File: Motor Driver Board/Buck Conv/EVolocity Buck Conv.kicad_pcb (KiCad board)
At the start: 4 copper layers, 120 x 90 mm, 53 parts, among them J1 Screw_Terminal_01x02, J2 XT30, J3 Screw_Terminal_01x02, J4 Conn_01x04, U1 NRF24L01_Breakout, U2 LM2576HVT-5, U4 L298N

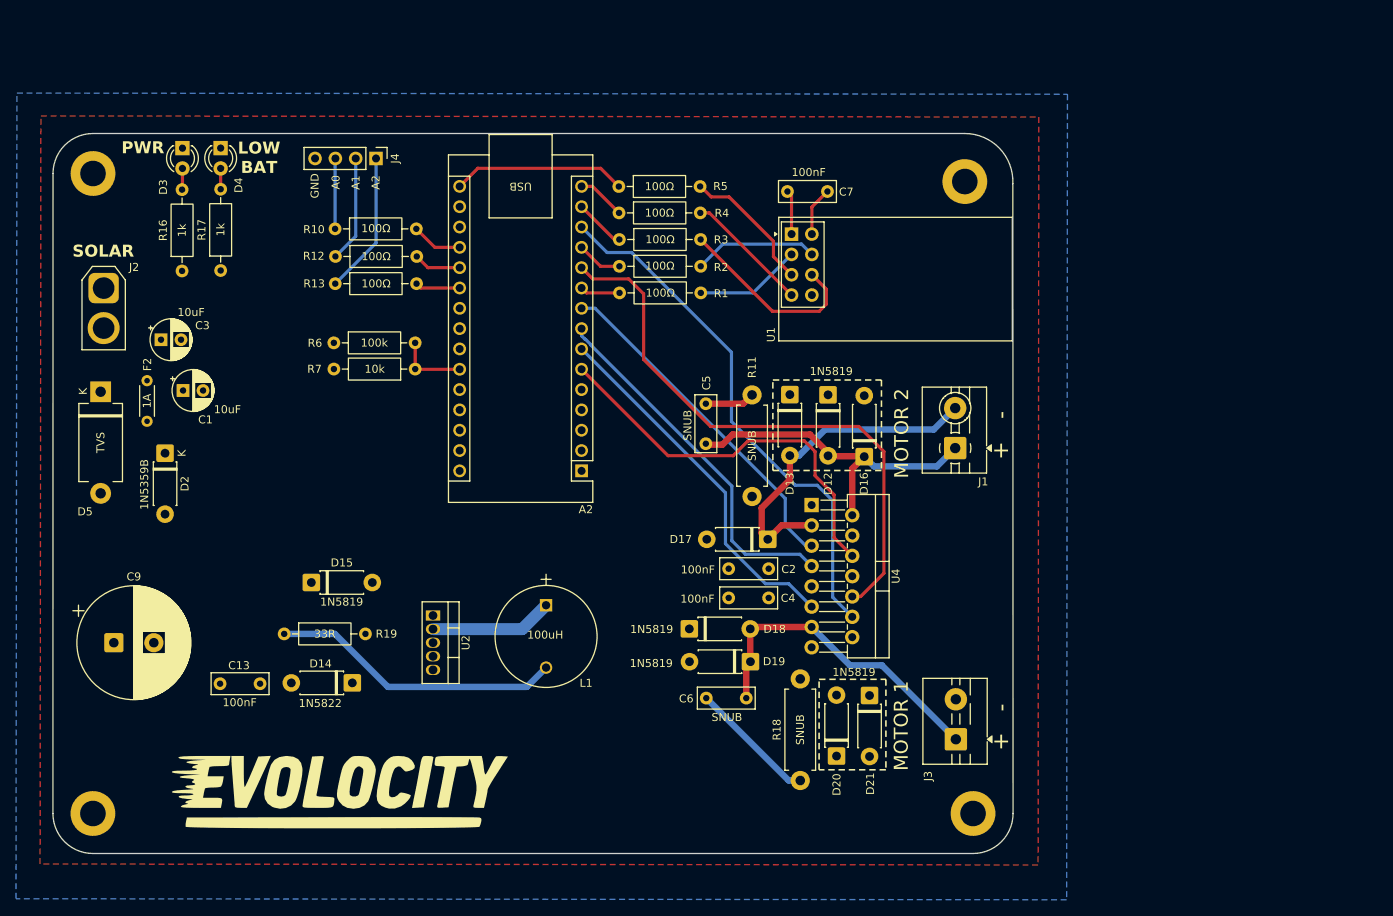
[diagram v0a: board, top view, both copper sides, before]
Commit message: updates after catchup
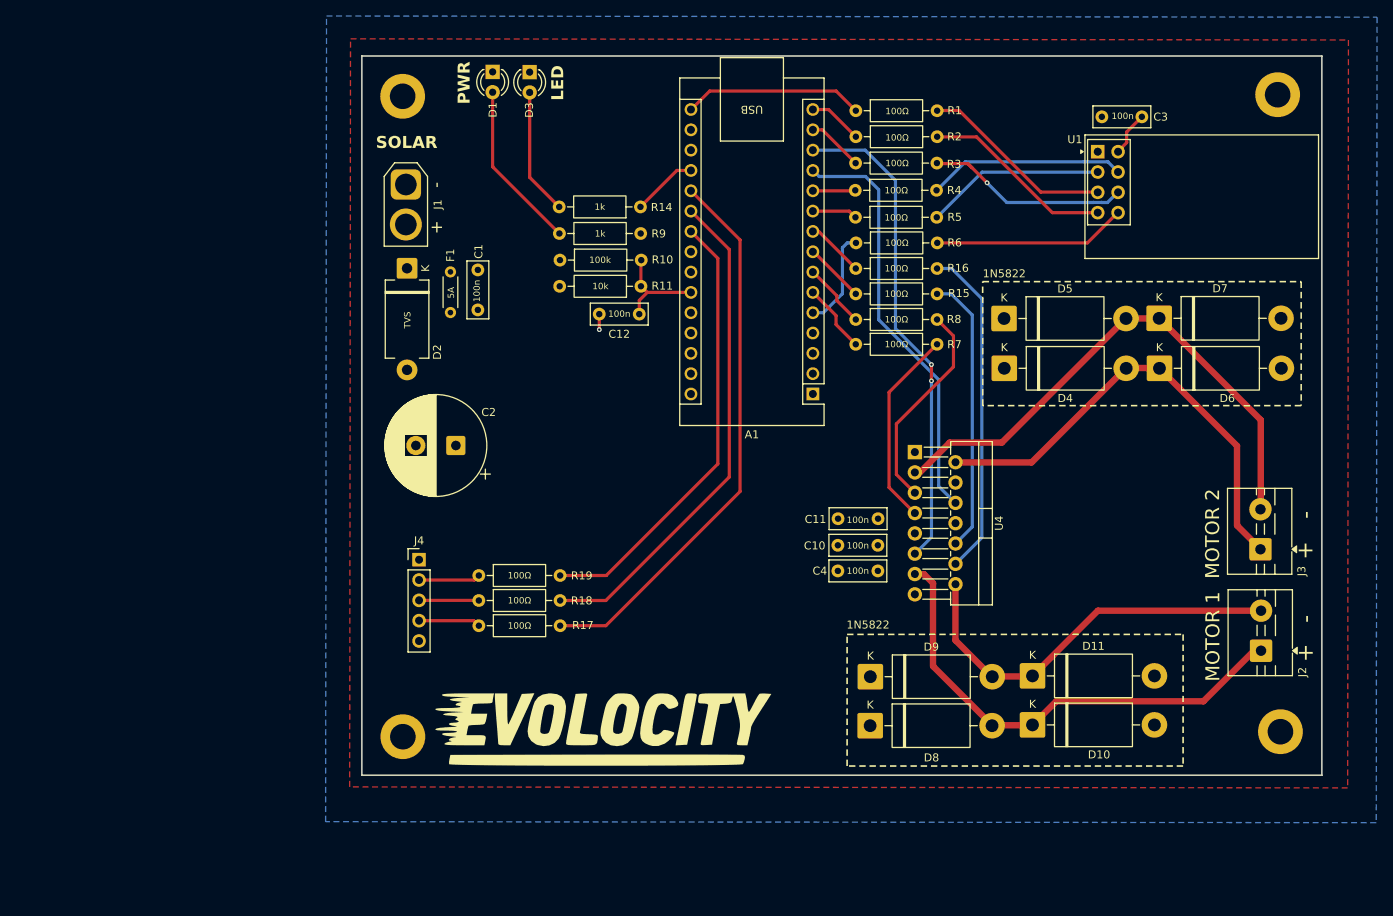
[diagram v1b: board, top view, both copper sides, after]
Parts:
- removed A2: Arduino_Nano_v3.x, Module:Arduino_Nano
- removed C13, C7: 100nF, Capacitor_THT:C_Rect_L7.0mm_W2.5mm_P5.00mm
- removed C5, C6: C_Snub, Capacitor_THT:C_Rect_L7.0mm_W2.5mm_P5.00mm
- removed C9: 100m, Capacitor_THT:CP_Radial_D14.0mm_P5.00mm
- removed D12, D13, D15, D16, D17, D18, D19, D20, D21: 1N5819, Diode_THT:D_DO-41_SOD81_P7.62mm_Horizontal
- removed D14: 1N5822, Diode_THT:D_DO-41_SOD81_P7.62mm_Horizontal
- removed F2: 1A, Resistor_THT:R_Axial_DIN0204_L3.6mm_D1.6mm_P5.08mm_Horizontal
- removed L1: 100uH, Library1:IND_BOURNS_RLB1314
- removed R12, R13: 100, Resistor_THT:R_Axial_DIN0207_L6.3mm_D2.5mm_P10.16mm_Horizontal
- removed U2: LM2576HVT-5, Package_TO_SOT_THT:TO-220-5_Vertical
- added A1: Arduino Nano, Module:Arduino_Nano, F.Cu at (136.0, 98.3)
- added C10: 100nF, Capacitor_THT:C_Rect_L7.0mm_W2.5mm_P5.00mm, F.Cu at (144.1, 117.2)
- added C11: 100nF, Capacitor_THT:C_Rect_L7.0mm_W2.5mm_P5.00mm, F.Cu at (144.1, 113.9)
- added C12: 100nF, Capacitor_THT:C_Rect_L7.0mm_W2.5mm_P5.00mm, F.Cu at (114.3, 88.3)
- added D1: Green, LED_THT:LED_D3.0mm_FlatTop, F.Cu at (96.0, 58.0)
- added D10: 1N5822, Diode_THT:D_DO-201AD_P15.24mm_Horizontal, F.Cu at (163.4, 139.7)
- added D11: 1N5822, Diode_THT:D_DO-201AD_P15.24mm_Horizontal, F.Cu at (163.4, 133.6)
- added D6: 1N5822, Diode_THT:D_DO-201AD_P15.24mm_Horizontal, F.Cu at (179.3, 95.1)
- added D7: 1N5822, Diode_THT:D_DO-201AD_P15.24mm_Horizontal, F.Cu at (179.3, 88.8)
- added D8: 1N5822, Diode_THT:D_DO-201AD_P15.24mm_Horizontal, F.Cu at (143.1, 139.8)
- added D9: 1N5822, Diode_THT:D_DO-201AD_P15.24mm_Horizontal, F.Cu at (143.2, 133.7)
- added F1: 5A, Resistor_THT:R_Axial_DIN0204_L3.6mm_D1.6mm_P5.08mm_Horizontal, F.Cu at (90.7, 83.0)
- added R14: 1k, Resistor_THT:R_Axial_DIN0207_L6.3mm_D2.5mm_P10.16mm_Horizontal, F.Cu at (114.4, 74.9)
- added R15: 100R, Resistor_THT:R_Axial_DIN0207_L6.3mm_D2.5mm_P10.16mm_Horizontal, F.Cu at (141.3, 85.8)
- added R8: 100R, Resistor_THT:R_Axial_DIN0207_L6.3mm_D2.5mm_P10.16mm_Horizontal, F.Cu at (141.3, 89.0)
- added R9: 1k, Resistor_THT:R_Axial_DIN0207_L6.3mm_D2.5mm_P10.16mm_Horizontal, F.Cu at (114.5, 78.2)
- C1, C3: value 10uF -> 100nF; footprint Capacitor_THT:CP_Radial_D5.0mm_P2.50mm -> Capacitor_THT:C_Rect_L7.0mm_W2.5mm_P5.00mm
- C2: value 100nF -> 470uF; footprint Capacitor_THT:C_Rect_L7.0mm_W2.5mm_P5.00mm -> Capacitor_THT:CP_Radial_D12.5mm_P5.00mm
- D2: value 1N5359B -> 1.5KE39CA (TVS); footprint Diode_THT:D_DO-41_SOD81_P7.62mm_Horizontal -> Diode_THT:D_DO-201_P12.70mm_Horizontal
- D4: value Red -> 1N5822; footprint LED_THT:LED_D3.0mm_FlatTop -> Diode_THT:D_DO-201AD_P15.24mm_Horizontal
- D5: value 1.5KE39CA (TVS) -> 1N5822; footprint Diode_THT:D_DO-201_P12.70mm_Horizontal -> Diode_THT:D_DO-201AD_P15.24mm_Horizontal
- J1: value Screw_Terminal_01x02 -> XT30; footprint TerminalBlock:TerminalBlock_MaiXu_MX126-5.0-02P_1x02_P5.00mm -> Connector_AMASS:AMASS_XT30U-F_1x02_P5.0mm_Vertical
- J2: value XT30 -> Screw_Terminal_01x02; footprint Connector_AMASS:AMASS_XT30U-F_1x02_P5.0mm_Vertical -> TerminalBlock:TerminalBlock_MaiXu_MX126-5.0-02P_1x02_P5.00mm
- J4: value Conn_01x04 -> Conn_01x05; footprint Connector_PinHeader_2.54mm:PinHeader_1x04_P2.54mm_Vertical -> Connector_PinHeader_2.54mm:PinHeader_1x05_P2.54mm_Vertical
- R1, R2, R3, R4, R5: value 100 -> 100R
- R10: value 100 -> 100k
- R11: value R_snub -> 10k; footprint Resistor_THT:R_Axial_DIN0411_L9.9mm_D3.6mm_P12.70mm_Horizontal -> Resistor_THT:R_Axial_DIN0207_L6.3mm_D2.5mm_P10.16mm_Horizontal
- R16, R17: value 1k -> 100R
- R18: value R_snub -> 100R; footprint Resistor_THT:R_Axial_DIN0411_L9.9mm_D3.6mm_P12.70mm_Horizontal -> Resistor_THT:R_Axial_DIN0207_L6.3mm_D2.5mm_P10.16mm_Horizontal
- R19: value 33R -> 100R
- R6: value 100k -> 100R
- R7: value 10k -> 100R
- moved J2 151.6 mm to (192.0, 130.4), turned to 90 degrees
- moved C3 125.7 mm to (177.1, 63.7), turned to 180 degrees
- moved D5 113.3 mm to (159.9, 88.9), turned to 0 degrees
- moved D4 101.7 mm to (159.9, 95.1), turned to 0 degrees
- moved H3 97.6 mm to (194.1, 60.9)
- moved R16 84.2 mm to (141.3, 82.6), turned to 0 degrees
- moved H4 79.3 mm to (194.4, 140.5)
- moved J1 76.2 mm to (85.1, 72.1), turned to -90 degrees
- moved R6 66.5 mm to (141.4, 79.4)
- moved R7 55.2 mm to (141.3, 92.1), turned to 0 degrees
- moved R17 54.9 mm to (94.2, 127.3), turned to 0 degrees
- moved J4 50.4 mm to (86.8, 119.0), turned to 0 degrees
- moved R18 46.1 mm to (94.2, 124.1), turned to 0 degrees
- moved J3 44.9 mm to (191.9, 117.7)
- moved D3 44.4 mm to (100.6, 58.1)
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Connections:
- C1 pad 1: +5V -> PowerInput+
- C2 pad 1: +5V -> PowerInput+
- C4 pad 1: +5V -> PowerInput+
- D2 pad 1: +5V -> PowerInput+
- D4 pad 1: GND -> PowerInput+
- D5 pad 1: Net-(D5-A1) -> PowerInput+
- D5 pad 2: GND -> Net-(D5-A)
- J1 pad 1: Net-(D12-A) -> GND
- J1 pad 2: Net-(D13-A) -> Net-(J1-Pin_2)
- J2 pad 1: GND -> Net-(D10-K)
- J2 pad 2: Net-(D5-A1) -> Net-(D11-K)
- J3 pad 1: Net-(D18-A) -> Net-(D4-A)
- J3 pad 2: Net-(D20-A) -> Net-(D5-A)
- J4 pad 1: /A2 -> GND
- J4 pad 2: /A1 -> /A3
- J4 pad 3: /A0 -> /A2
- J4 pad 4: GND -> /A1
- R1 pad 2: /Radio_CE -> /Radio_SCK
- R10 pad 1: /A0 -> PowerInput+
- R10 pad 2: Net-(A2-A0) -> /V_Panel_Analog
- R11 pad 1: Net-(C5-Pad2) -> /V_Panel_Analog
- R11 pad 2: Net-(D13-A) -> GND
- R16 pad 1: +5V -> Net-(A1-D6)
- R16 pad 2: Net-(D3-A) -> /Motor_IN4
- R17 pad 1: /LowBattLED -> /A1
- R17 pad 2: Net-(D4-A) -> Net-(A1-A1)
- R18 pad 1: Net-(C6-Pad2) -> /A2
- R18 pad 2: Net-(D20-A) -> Net-(A1-A2)
- R19 pad 1: Net-(L1-Pad2) -> /A3
- R2 pad 2: /Radio_CS -> /Radio_MISO
- R4 pad 2: /Radio_MISO -> /Radio_CS
- R5 pad 2: /Radio_SCK -> /Radio_CE
- R6 pad 1: +5V -> Net-(A1-D2)
- R6 pad 2: /V_Panel_Analog -> /Radio_IRQ
- R7 pad 1: /V_Panel_Analog -> Net-(A1-D3)
- R7 pad 2: GND -> /Motor_IN2
- U1 pad 2: +3V3 -> +5V
- U1 pad 8: unconnected-(U1-IRQ-Pad8) -> /Radio_IRQ
- U4 pad 10: /IN3 -> /Motor_IN3
- U4 pad 11: /EnB -> /Motor_EnB
- U4 pad 12: /IN4 -> /Motor_IN4
- U4 pad 13: Net-(D18-A) -> Net-(D10-K)
- U4 pad 14: Net-(D20-A) -> Net-(D11-K)
- U4 pad 2: Net-(D12-A) -> Net-(D4-A)
- U4 pad 3: Net-(D13-A) -> Net-(D5-A)
- U4 pad 4: +5V -> PowerInput+
- U4 pad 5: /IN1 -> /Motor_IN1
- U4 pad 6: /EnA -> /Motor_EnA
- U4 pad 7: /IN2 -> /Motor_IN2
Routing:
- net PowerInput+: track 0.00 -> 207.1 mm
- net +5V: track 105.1 -> 13.6 mm
- net /IN3: track 72.5 -> 0.00 mm
- net Net-(A1-A1): track 0.00 -> 69.6 mm
- net Net-(D5-A): track 0.00 -> 67.6 mm
- net /IN4: track 66.2 -> 0.00 mm
- net Net-(A1-A2): track 0.00 -> 62.8 mm
- net /Motor_EnB: track 0.00 -> 61.3 mm, vias 0 -> 2
- net Net-(D10-K): track 0.00 -> 61.0 mm
- net Net-(D4-A): track 2.60 -> 58.3 mm
- net /Motor_EnA: track 0.00 -> 52.3 mm
- net Net-(D11-K): track 0.00 -> 50.6 mm
- net /EnA: track 49.9 -> 0.00 mm
- net Net-(A1-A3): track 6.78 -> 56.0 mm
- net /EnB: track 45.8 -> 0.00 mm
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- removed copper zone on In2.Cu, net +3V3
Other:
- board size 120 x 90 mm -> 120 x 89.9 mm
- board text added: "100n"
- board text added: "5A"
- board text added: "LED"
- board text removed: "100nF"
- board text removed: "100uH"
- board text removed: "10uF"
- board text removed: "1A"
- board text removed: "1N5359B"
- board text removed: "1N5819"
- board text removed: "33R"
- board text removed: "A0"
- board text removed: "A1"
- board text removed: "A2"
- board text removed: "GND"
- board text removed: "LOW BAT"
- board text removed: "SNUB"
